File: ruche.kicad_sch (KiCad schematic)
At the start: 32 parts, among them IC2 MAX17048G+, IC3 L86-M33, IC4 SHT41-AD1B-R3, J13 Micro_SD_Card, U1 MKRWAN_1310, U2 MS5611-01BA, U3 XC6220B331MR

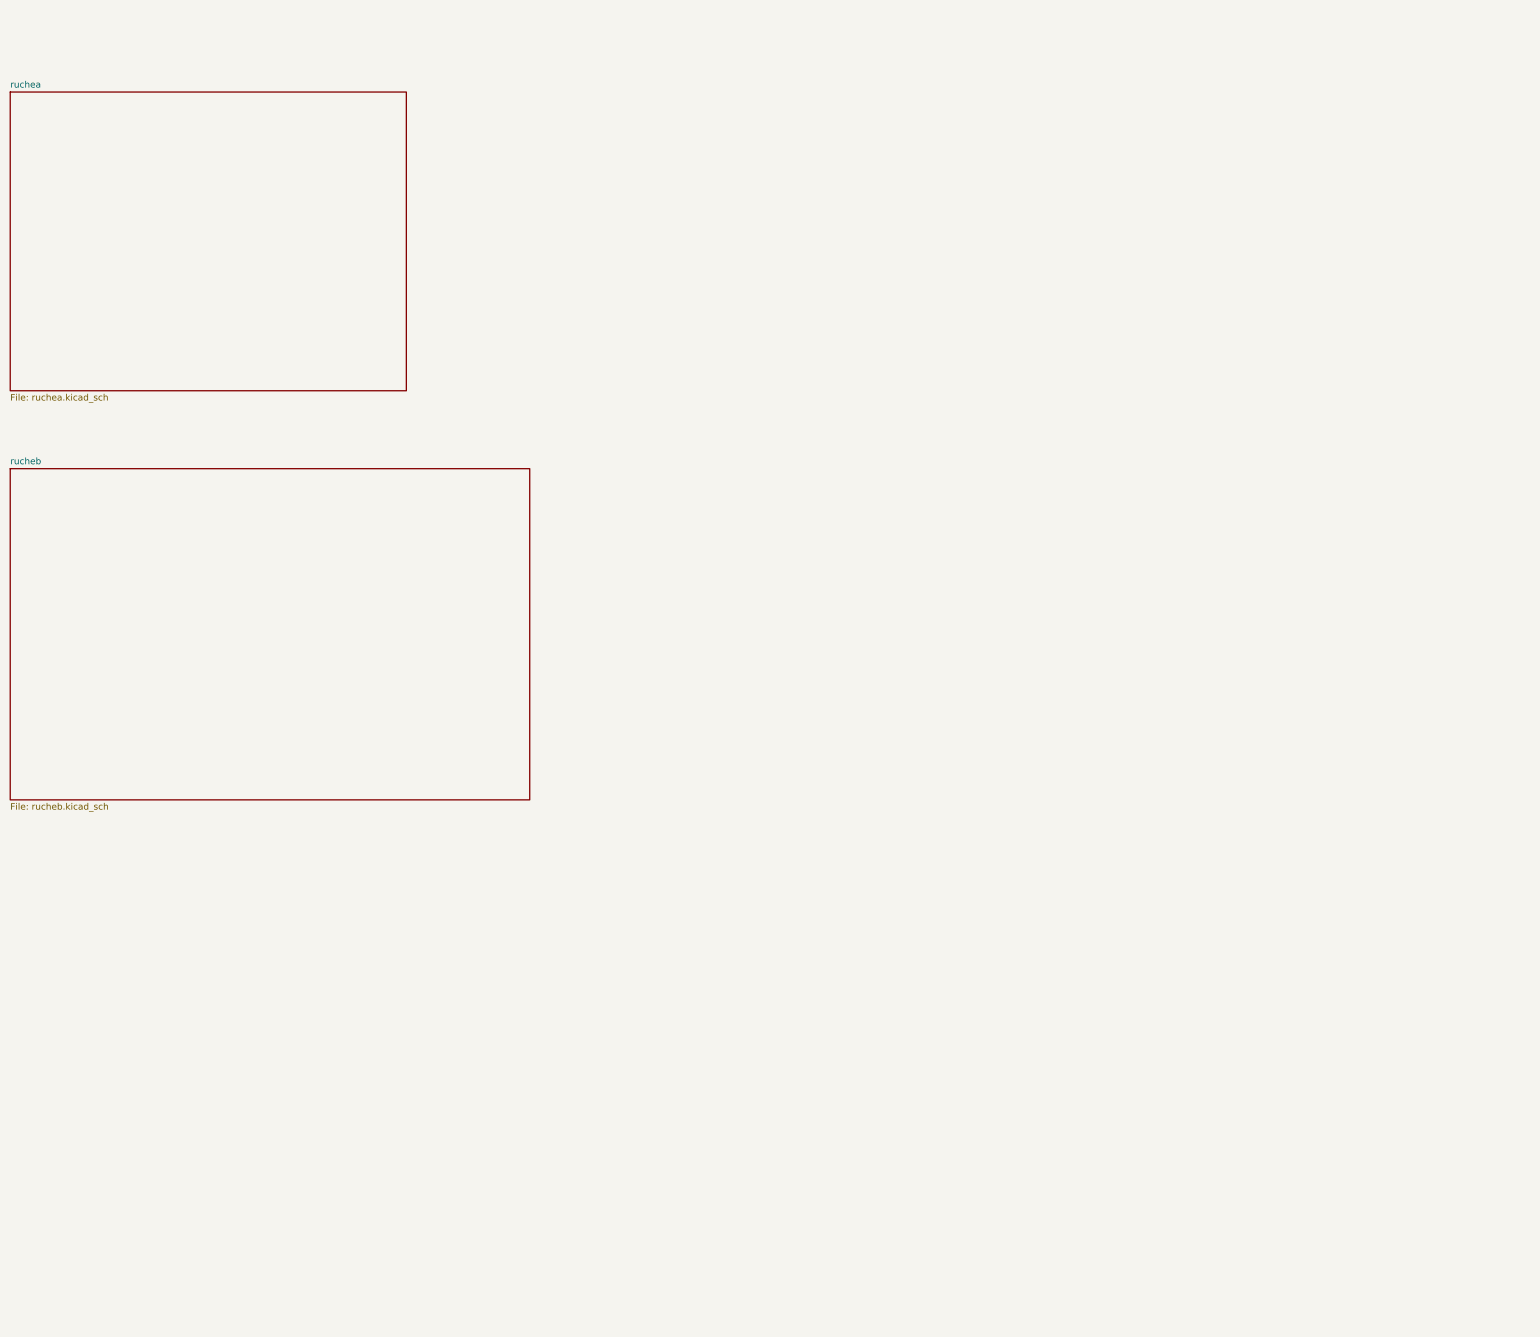
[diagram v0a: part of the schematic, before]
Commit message: Add graphics
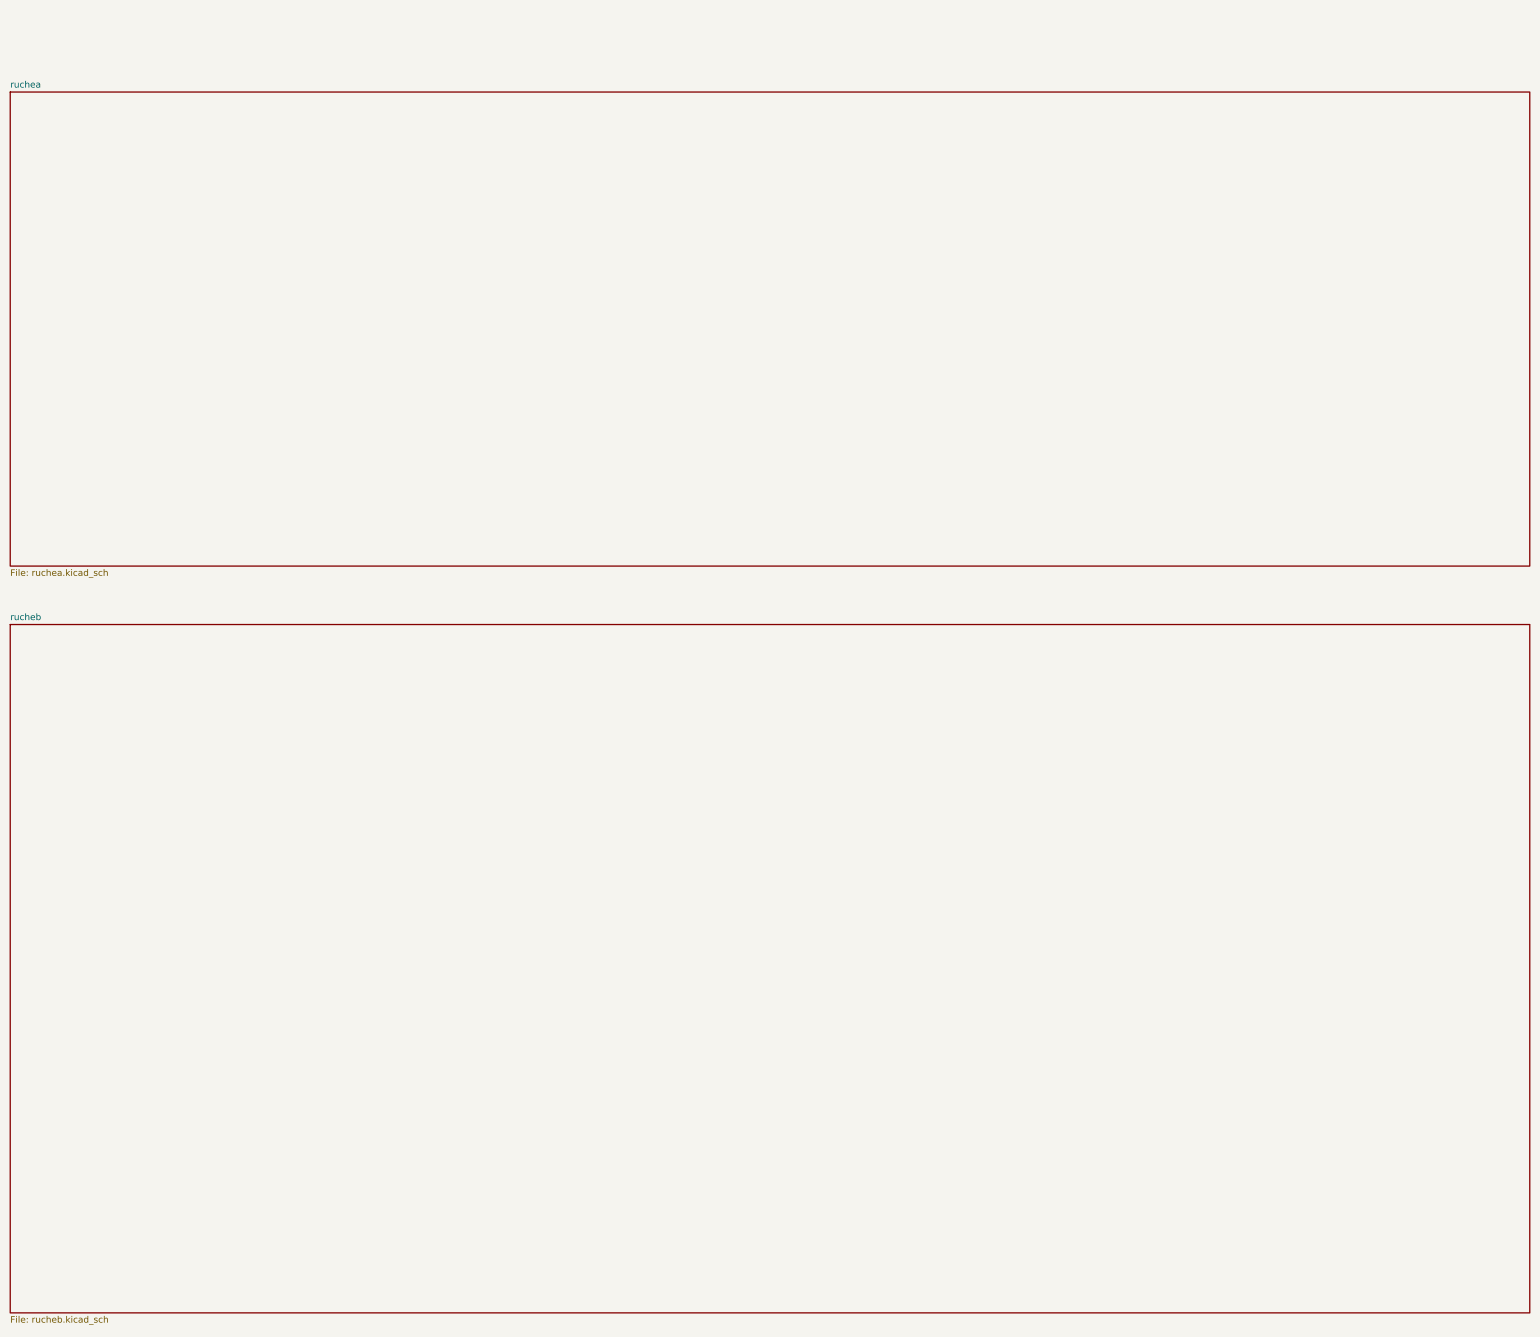
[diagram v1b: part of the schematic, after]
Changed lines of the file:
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@@
     (pin "2")
   )
-  (sheet (at 0 215.9) (size 77.47 58.42) (fields_autoplaced)
+  (sheet (at 0 215.9) (size 297.18 92.71) (fields_autoplaced)
     (stroke (width 0) (type solid) (color 0 0 0 0))
     (fill (color 0 0 0 0.0000))
@@
       (effects (font (size 1.27 1.27)) (justify left bottom))
     )
-    (property "Sheet file" "ruchea.kicad_sch" (id 1) (at 0 274.9046 0)
+    (property "Sheet file" "ruchea.kicad_sch" (id 1) (at 0 309.1946 0)
       (effects (font (size 1.27 1.27)) (justify left top))
     )
   )
-  (sheet (at 0 289.56) (size 101.6 64.77) (fields_autoplaced)
+  (sheet (at 0 320.04) (size 297.18 134.62) (fields_autoplaced)
     (stroke (width 0) (type solid) (color 0 0 0 0))
     (fill (color 0 0 0 0.0000))
-    (property "Sheet name" "rucheb" (id 0) (at 0 288.8484 0)
+    (property "Sheet name" "rucheb" (id 0) (at 0 319.3284 0)
       (effects (font (size 1.27 1.27)) (justify left bottom))
     )
-    (property "Sheet file" "rucheb.kicad_sch" (id 1) (at 0 354.9146 0)
+    (property "Sheet file" "rucheb.kicad_sch" (id 1) (at 0 455.2446 0)
       (effects (font (size 1.27 1.27)) (justify left top))
     )
